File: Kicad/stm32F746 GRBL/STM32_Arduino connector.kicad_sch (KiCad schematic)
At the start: 9 parts, among them CN1 PinHeader_1x08_P2.54mm_Vertic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, CN2 PinHeader_1x06_P2.54mm_Vertic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, CN3 PinHeader_1x10_P2.54mm_Vertic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, CN4 PinHeader_1x08_P2.54mm_Vertic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, U3 24LC64

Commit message: wip kicad
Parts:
- RN1: footprint Package_SO:SOIC-16W-12_7.5x10.3mm_P1.27mm -> Package_SO:SOIC-16W_5.3x10.2mm_P1.27mm
- RN2, RN3: footprint (none) -> Package_SO:SOIC-16W_5.3x10.2mm_P1.27mm
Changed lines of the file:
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@@
       (effects (font (size 1.27 1.27)))
     )
-    (property "Footprint" "" (at 134.62 92.075 90)
+    (property "Footprint" "Package_SO:SOIC-16W_5.3x10.2mm_P1.27mm" (at 134.62 92.075 90)
       (effects (font (size 1.27 1.27)) hide)
     )
@@
       (effects (font (size 1.27 1.27)))
     )
-    (property "Footprint" "" (at 134.62 69.215 90)
+    (property "Footprint" "Package_SO:SOIC-16W_5.3x10.2mm_P1.27mm" (at 134.62 69.215 90)
       (effects (font (size 1.27 1.27)) hide)
     )
@@
       (effects (font (size 1.27 1.27)))
     )
-    (property "Footprint" "Package_SO:SOIC-16W-12_7.5x10.3mm_P1.27mm" (at 86.36 92.075 90)
-      (effects (font (size 1.27 1.27)) hide)
-    )
+    (property "Footprint" "Package_SO:SOIC-16W_5.3x10.2mm_P1.27mm" (at 86.36 92.075 90)
+      (effects (font (size 1.27 1.27)) hide)
+    )

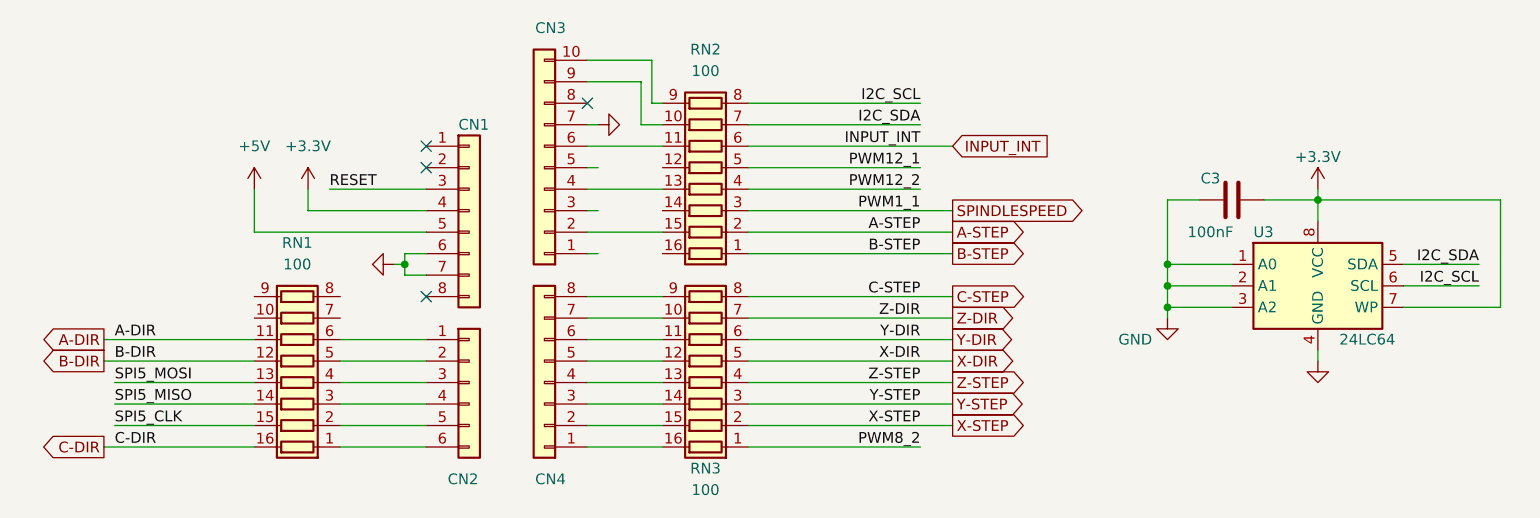
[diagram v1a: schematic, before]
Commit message: wip
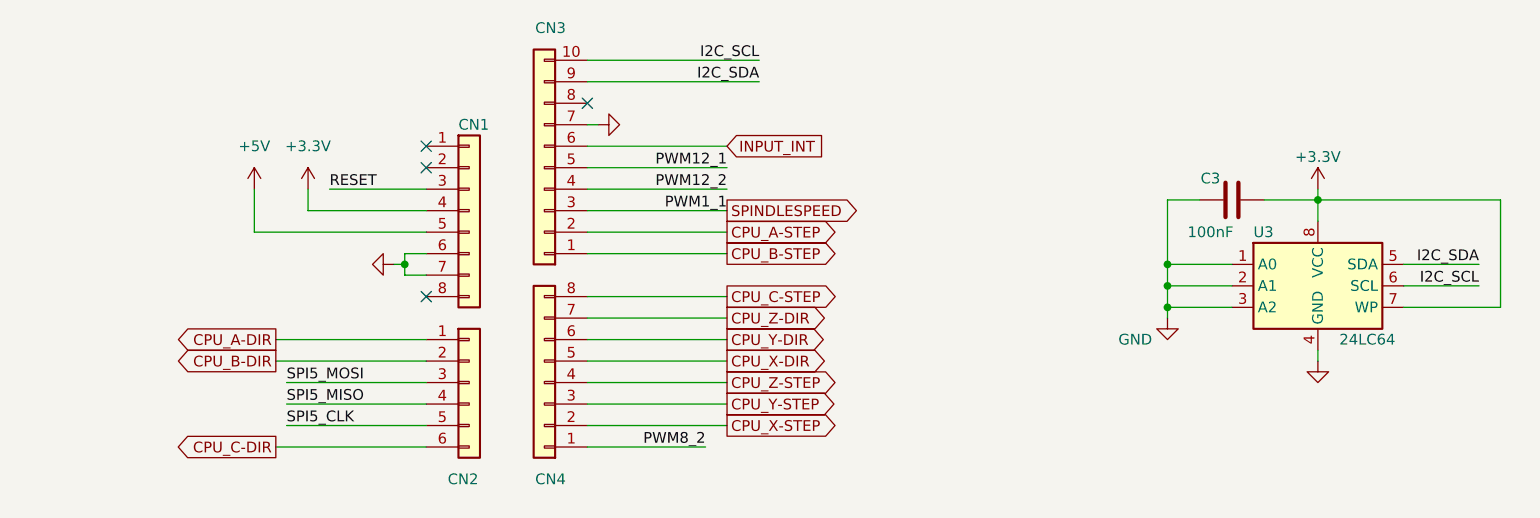
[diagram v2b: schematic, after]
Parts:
- removed RN1, RN2, RN3: 100, Package_SO:SOIC-16W_5.3x10.2mm_P1.27mm, symbol Device:R_Pack08
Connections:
- net I2C_SCL: now also CN3.10 (Pin_10)
- net I2C_SDA: now also CN3.9 (Pin_9)
- net INPUT_INT: now also CN3.6 (Pin_6)
- net PWM12_1: now also CN3.5 (Pin_5)
- net PWM12_2: now also CN3.4 (Pin_4)
- net PWM8_2: now also CN4.1 (Pin_1)
- net SPI5_CLK: now also CN2.5 (Pin_5)
- net SPI5_MISO: now also CN2.4 (Pin_4)
- net SPI5_MOSI: now also CN2.3 (Pin_3)
- net SPINDLESPEED: now also CN3.3 (Pin_3)
- net CPU_X-STEP: now reaches CN4.2 (Pin_2)
- net CPU_Y-STEP: now reaches CN4.3 (Pin_3)
- net CPU_Z-STEP: now reaches CN4.4 (Pin_4)
- net CPU_X-DIR: now reaches CN4.5 (Pin_5)
- net CPU_Y-DIR: now reaches CN4.6 (Pin_6)
- net CPU_Z-DIR: now reaches CN4.7 (Pin_7)
- net CPU_C-STEP: now reaches CN4.8 (Pin_8)
- net CPU_A-DIR: now reaches CN2.1 (Pin_1)
- net CPU_B-DIR: now reaches CN2.2 (Pin_2)
- net CPU_C-DIR: now reaches CN2.6 (Pin_6)
- net CPU_A-STEP: now reaches CN3.2 (Pin_2)
- net CPU_B-STEP: now reaches CN3.1 (Pin_1)

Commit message: wip Kicad
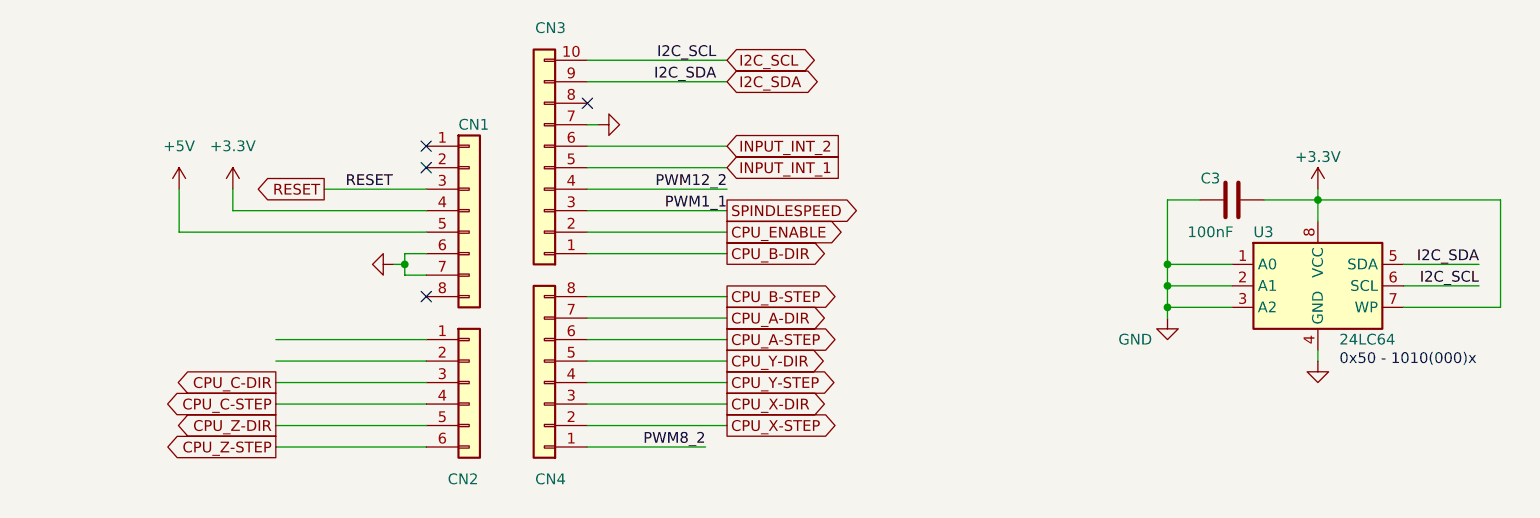
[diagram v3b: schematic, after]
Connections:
- net SPI5_CLK is gone; now on net CPU_Z-DIR: CN2.5 (Pin_5)
- net SPI5_MISO is gone; now on net CPU_C-STEP: CN2.4 (Pin_4)
- net SPI5_MOSI is gone; now on net CPU_C-DIR: CN2.3 (Pin_3)
- net CPU_A-DIR: now also CN4.7 (Pin_7); no longer CN2.1 (Pin_1)
- net CPU_A-STEP: now also CN4.6 (Pin_6); no longer CN3.2 (Pin_2)
- net CPU_B-DIR: now also CN3.1 (Pin_1); no longer CN2.2 (Pin_2)
- net CPU_B-STEP: now also CN4.8 (Pin_8); no longer CN3.1 (Pin_1)
- net CPU_C-DIR: no longer CN2.6 (Pin_6)
- net CPU_C-STEP: no longer CN4.8 (Pin_8)
- net CPU_X-DIR: now also CN4.3 (Pin_3); no longer CN4.5 (Pin_5)
- net CPU_Y-DIR: now also CN4.5 (Pin_5); no longer CN4.6 (Pin_6)
- net CPU_Y-STEP: now also CN4.4 (Pin_4); no longer CN4.3 (Pin_3)
- net CPU_Z-DIR: no longer CN4.7 (Pin_7)
- net CPU_Z-STEP: now also CN2.6 (Pin_6); no longer CN4.4 (Pin_4)
- net INPUT_INT renamed INPUT_INT_2
- net PWM12_1 renamed INPUT_INT_1
- new net CPU_ENABLE: CN3.2 (Pin_2)
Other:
- note added: "0x50 - 1010(000)x"

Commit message: kicad wip
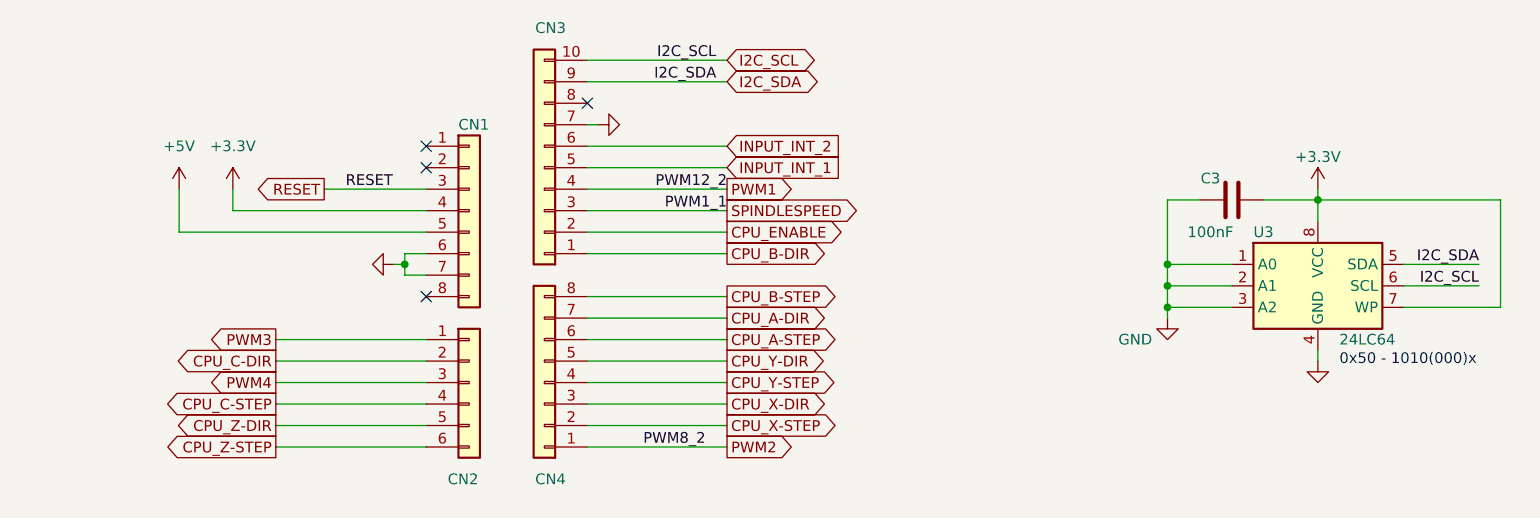
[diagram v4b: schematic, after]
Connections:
- net CPU_C-DIR: now also CN2.2 (Pin_2); no longer CN2.3 (Pin_3)
- net PWM3: now reaches CN2.1 (Pin_1)
- net PWM12_2 renamed PWM1
- net PWM8_2 renamed PWM2
- new net PWM4: CN2.3 (Pin_3)
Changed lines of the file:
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@@
     (stroke (width 0) (type default))
   )
-  (wire (pts (xy 120.65 114.3) (xy 134.62 114.3))
+  (wire (pts (xy 120.65 114.3) (xy 137.16 114.3))
     (stroke (width 0) (type default))
   )
@@
     )
   )
+  (global_label "PWM1" (shape output) (at 137.16 83.82 0) (fields_autoplaced)
+    (effects (font (size 1.27 1.27)) (justify left))
+    (property "Intersheetrefs" "${INTERSHEET_REFS}" (at 145.5275 83.82 0)
+      (effects (font (size 1.27 1.27)) (justify left) hide)
+    )
+  )
+  (global_label "CPU_C-DIR" (shape output) (at 83.82 104.14 180) (fields_autoplaced)
+    (effects (font (size 1.27 1.27)) (justify right))
+    (property "Intersheetrefs" "${INTERSHEET_REFS}" (at 70.0095 104.14 0)
+      (effects (font (size 1.27 1.27)) (justify right) hide)
+    )
+  )
   (global_label "I2C_SCL" (shape bidirectional) (at 137.16 68.58 0) (fields_autoplaced)
     (effects (font (size 1.27 1.27)) (justify left))
@@
     )
   )
-  (global_label "CPU_C-DIR" (shape output) (at 83.82 106.68 180) (fields_autoplaced)
+  (global_label "PWM2" (shape output) (at 137.16 114.3 0) (fields_autoplaced)
+    (effects (font (size 1.27 1.27)) (justify left))
+    (property "Intersheetrefs" "${INTERSHEET_REFS}" (at 145.5275 114.3 0)
+      (effects (font (size 1.27 1.27)) (justify left) hide)
+    )
+  )
+  (global_label "PWM4" (shape output) (at 83.82 106.68 180) (fields_autoplaced)
     (effects (font (size 1.27 1.27)) (justify right))
-    (property "Intersheetrefs" "${INTERSHEET_REFS}" (at 70.0095 106.68 0)
+    (property "Intersheetrefs" "${INTERSHEET_REFS}" (at 75.4525 106.68 0)
       (effects (font (size 1.27 1.27)) (justify right) hide)
     )
@@
     )
   )
+  (global_label "PWM3" (shape output) (at 83.82 101.6 180) (fields_autoplaced)
+    (effects (font (size 1.27 1.27)) (justify right))
+    (property "Intersheetrefs" "${INTERSHEET_REFS}" (at 75.4525 101.6 0)
+      (effects (font (size 1.27 1.27)) (justify right) hide)
+    )
+  )

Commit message: wip kicad
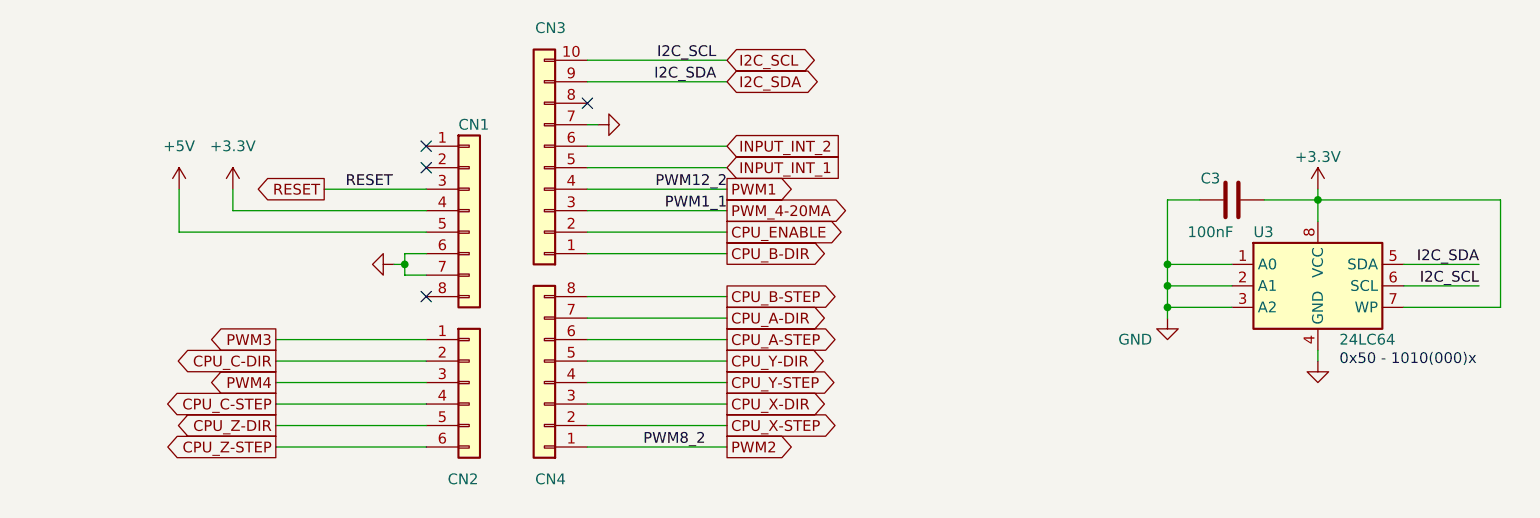
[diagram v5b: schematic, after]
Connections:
- net SPINDLESPEED renamed PWM_4-20MA
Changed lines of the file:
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@@
     )
   )
-  (global_label "SPINDLESPEED" (shape output) (at 137.16 86.36 0) (fields_autoplaced)
+  (global_label "PWM_4-20MA" (shape output) (at 137.16 86.36 0) (fields_autoplaced)
     (effects (font (size 1.27 1.27)) (justify left))
-    (property "Intersheetrefs" "${INTERSHEET_REFS}" (at 154.0546 86.36 0)
+    (property "Intersheetrefs" "${INTERSHEET_REFS}" (at 153.0265 86.36 0)
       (effects (font (size 1.27 1.27)) (justify left) hide)
     )
